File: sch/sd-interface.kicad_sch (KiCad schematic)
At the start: 33 parts, among them J15 F32Q-1A7H1-11022, J16 MEM2075-00-140-01-A, J17 5V_out, J19 3V3_in, Q1 Q_PMOS_GSD, U10 CD4043BDR, U11 TPS22919DCKR, U8 MAX4996LETG_

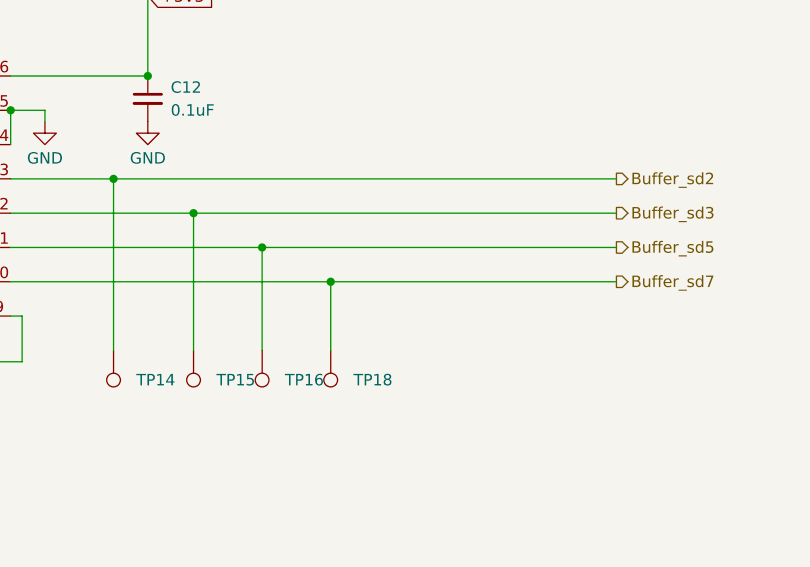
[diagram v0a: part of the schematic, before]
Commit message: earth plane, vias, connector ect
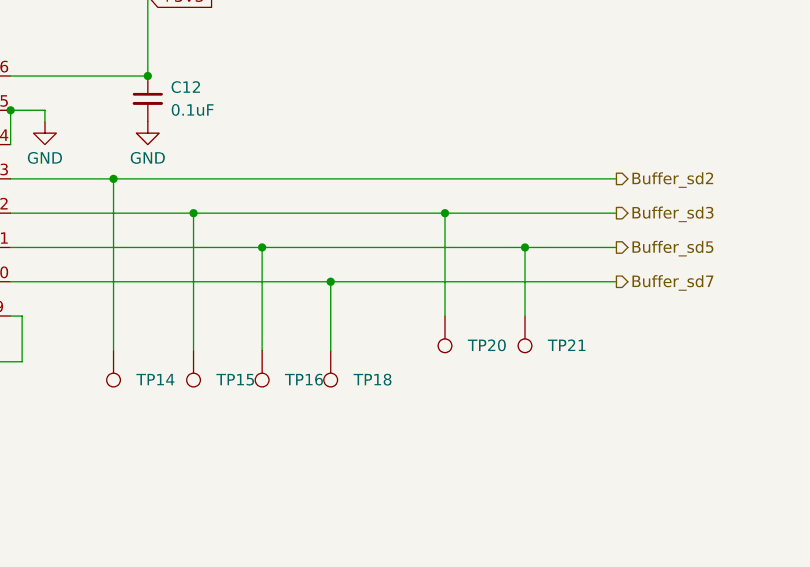
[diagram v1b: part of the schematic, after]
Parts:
- added TP20, TP21: TestPoint, TestPoint:TestPoint_Pad_D1.0mm, symbol Connector:TestPoint
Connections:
- net Buffer_sd3: now also TP20.1
- net Buffer_sd5: now also TP21.1
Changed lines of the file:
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@@
 	)
 	(junction
+		(at 255.27 58.42)
+		(diameter 0)
+		(color 0 0 0 0)
+	)
+	(junction
 		(at 182.88 74.93)
 		(diameter 0)
@@
 	)
 	(junction
+		(at 264.16 62.23)
+		(diameter 0)
+		(color 0 0 0 0)
+	)
+	(junction
 		(at 91.44 163.83)
 		(diameter 0)
@@
 	(wire
 		(pts
-			(xy 227.33 58.42) (xy 274.32 58.42)
+			(xy 227.33 58.42) (xy 255.27 58.42)
 		)
 		(stroke
@@
 	(wire
 		(pts
+			(xy 255.27 58.42) (xy 255.27 69.85)
+		)
+		(stroke
+			(width 0)
+			(type default)
+		)
+	)
+	(wire
+		(pts
 			(xy 50.8 41.91) (xy 50.8 68.58)
 		)
@@
 	(wire
 		(pts
+			(xy 264.16 62.23) (xy 274.32 62.23)
+		)
+		(stroke
+			(width 0)
+			(type default)
+		)
+	)
+	(wire
+		(pts
 			(xy 170.18 232.41) (xy 172.72 232.41)
 		)
@@
 	(wire
 		(pts
+			(xy 255.27 58.42) (xy 274.32 58.42)
+		)
+		(stroke
+			(width 0)
+			(type default)
+		)
+	)
+	(wire
+		(pts
 			(xy 144.78 62.23) (xy 144.78 66.04)
 		)
@@
 	(wire
 		(pts
-			(xy 234.95 62.23) (xy 274.32 62.23)
+			(xy 234.95 62.23) (xy 264.16 62.23)
 		)
 		(stroke
@@
 	(wire
 		(pts
+			(xy 264.16 62.23) (xy 264.16 69.85)
+		)
+		(stroke
+			(width 0)
+			(type default)
+		)
+	)
+	(wire
+		(pts
 			(xy 86.36 36.83) (xy 86.36 41.91)
 		)
@@
 	)
 	(symbol
+		(lib_id "Connector:TestPoint")
+		(at 264.16 69.85 180)
+		(unit 1)
+		(exclude_from_sim no)
+		(in_bom yes)
+		(on_board yes)
+		(dnp no)
+		(fields_autoplaced yes)
+		(property "Reference" "TP21"
+			(at 266.7 73.1519 0)
+			(effects
+				(font
+					(size 1.27 1.27)
+				)
+				(justify right)
+			)
+		)
+		(property "Value" "TestPoint"
+			(at 261.62 71.8821 0)
+			(effects
+				(font
+					(size 1.27 1.27)
+				)
+				(justify left)
+				(hide yes)
+			)
+		)
+		(property "Footprint" "TestPoint:TestPoint_Pad_D1.0mm"
+			(at 259.08 69.85 0)
+			(effects
+				(font
+					(size 1.27 1.27)
+				)
+				(hide yes)
+			)
+		)
+		(property "Datasheet" "~"
+			(at 259.08 69.85 0)
+			(effects
+				(font
+					(size 1.27 1.27)
+				)
+				(hide yes)
+			)
+		)
+		(property "Description" "test point"
+			(at 264.16 69.85 0)
+			(effects
+				(font
+					(size 1.27 1.27)
+				)
+				(hide yes)
+			)
+		)
+		(pin "1"
+		)
+		(instances
+			(project "audiograb"
+				(path "/c46c2311-6d4b-411d-b012-c7730eac136d/6c55ccce-577d-49c2-8294-3a5d8e11981e"
+					(reference "TP21")
+					(unit 1)
+				)
+			)
+		)
+	)
+	(symbol
 		(lib_id "power:GND")
 		(at 346.71 220.98 0)
@@
 					(unit 1)
 				)
+			)
+		)
+	)
+	(symbol
+		(lib_id "Connector:TestPoint")
+		(at 255.27 69.85 180)
+		(unit 1)
+		(exclude_from_sim no)
+		(in_bom yes)
+		(on_board yes)
+		(dnp no)
+		(fields_autoplaced yes)
+		(property "Reference" "TP20"
+			(at 257.81 73.1519 0)
+			(effects
+				(font
+					(size 1.27 1.27)
+				)
+				(justify right)
+			)
+		)
+		(property "Value" "TestPoint"
+			(at 252.73 71.8821 0)
+			(effects
+				(font
+					(size 1.27 1.27)
+				)
+				(justify left)
+				(hide yes)
+			)
+		)
+		(property "Footprint" "TestPoint:TestPoint_Pad_D1.0mm"
+			(at 250.19 69.85 0)
+			(effects
+				(font
+					(size 1.27 1.27)
+				)
+				(hide yes)
+			)
+		)
+		(property "Datasheet" "~"
+			(at 250.19 69.85 0)
+			(effects
+				(font
+					(size 1.27 1.27)
+				)
+				(hide yes)
+			)
+		)
+		(property "Description" "test point"
+			(at 255.27 69.85 0)
+			(effects
+				(font
+					(size 1.27 1.27)
+				)
+				(hide yes)
+			)
+		)
+		(pin "1"
+		)
+		(instances
+			(project "audiograb"
+				(path "/c46c2311-6d4b-411d-b012-c7730eac136d/6c55ccce-577d-49c2-8294-3a5d8e11981e"
+					(reference "TP20")
+					(unit 1)
+				)
